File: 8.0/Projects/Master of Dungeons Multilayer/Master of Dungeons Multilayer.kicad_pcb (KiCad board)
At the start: 4 copper layers, 100 x 100 mm, 124 parts, among them J1 AudioPlug3, Q1 IRLML6244, Q10 IRLML6244, Q11 IRLML6244, Q12 IRLML6244, Q13 IRLML6244, Q14 IRLML6244, Q15 IRLML6244, Q16 IRLML6244, Q17 IRLML6244, Q2 IRLML6244, Q3 IRLML6244, Q4 IRLML6244, Q5 IRLML6244, Q6 IRLML6244, Q7 IRLML6244, Q8 IRLML6244, Q9 IRLML6244, U1 ESP32-WROOM-32E, U2 TPS63060, U3 AP2127K-3.3, U4 TSOP45xx

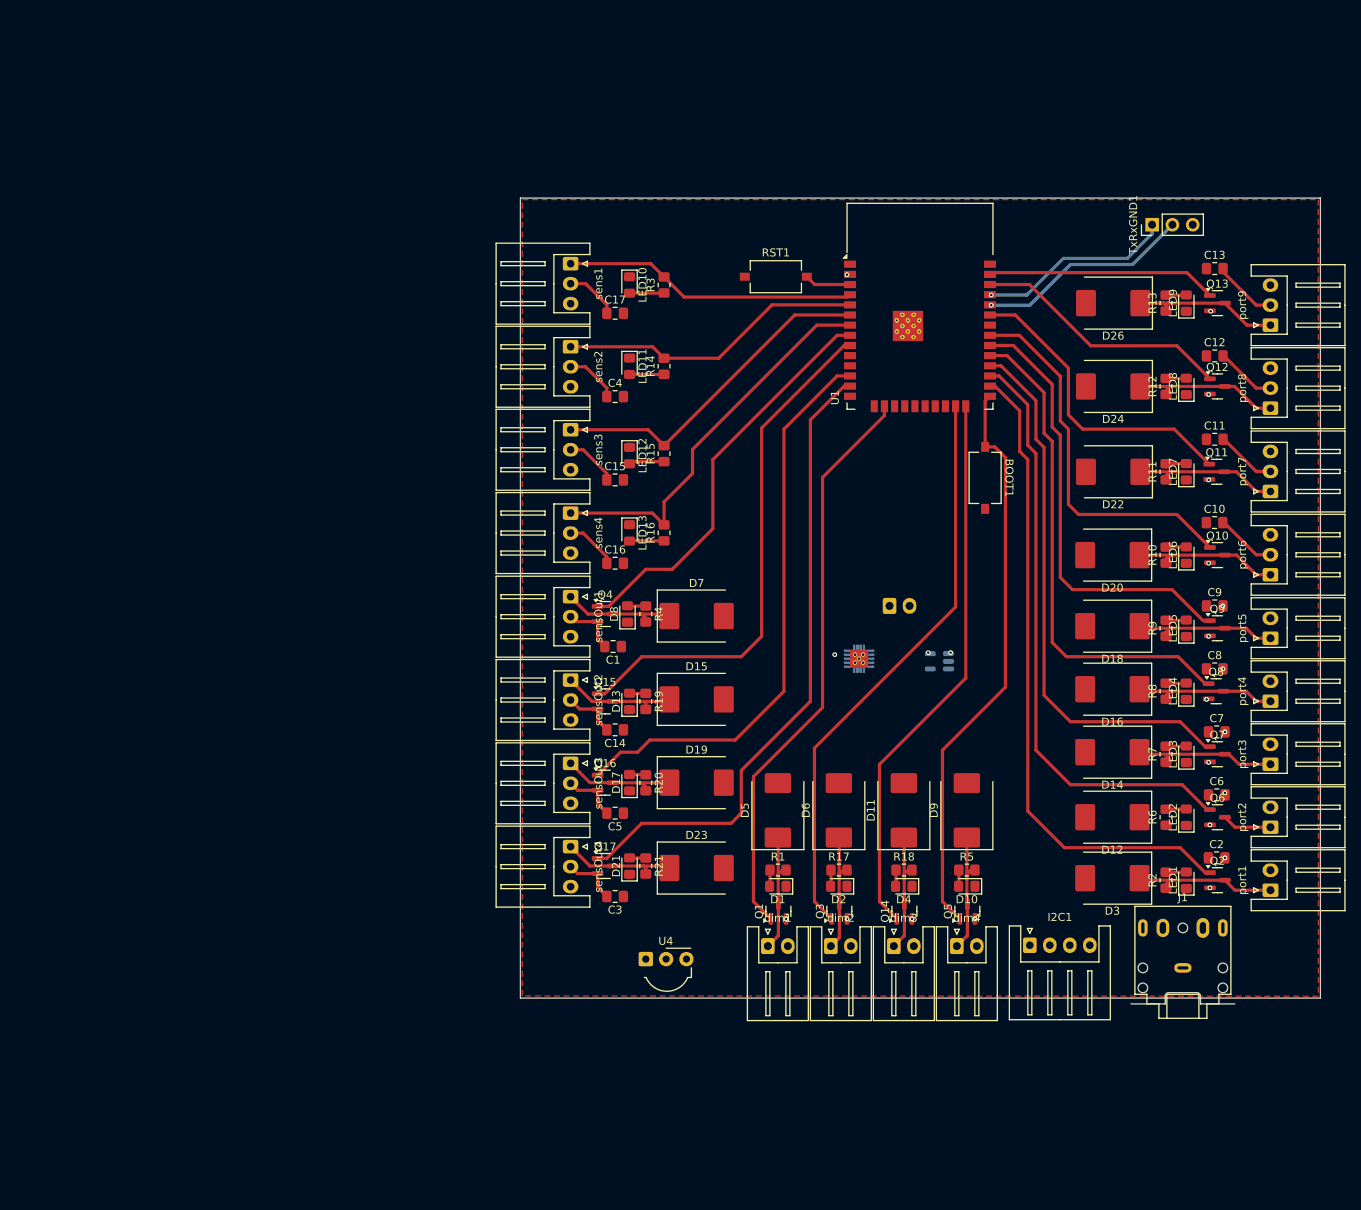
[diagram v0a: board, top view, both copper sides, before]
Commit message: update
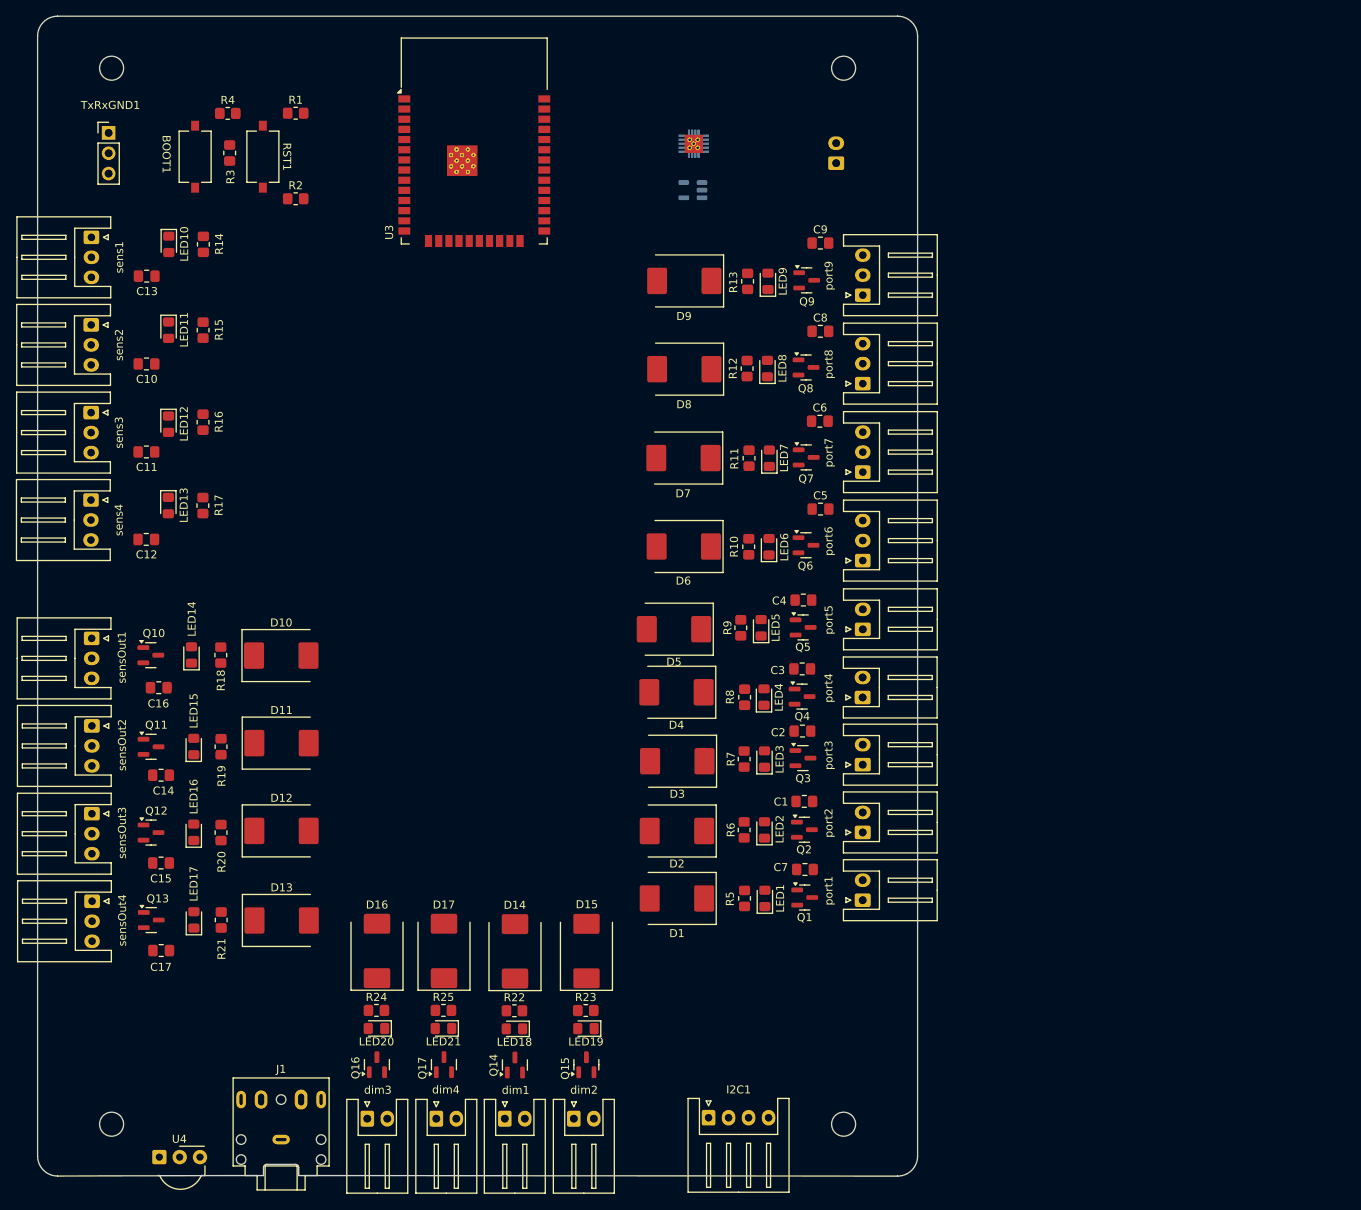
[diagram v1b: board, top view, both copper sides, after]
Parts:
- added R1: 470R, Resistor_SMD:R_0805_2012Metric_Pad1.20x1.40mm_HandSolder, F.Cu at (72.1, 39.5)
- added R2: 12K, Resistor_SMD:R_0805_2012Metric_Pad1.20x1.40mm_HandSolder, F.Cu at (72.1, 50.2)
- added R3: 12K, Resistor_SMD:R_0805_2012Metric_Pad1.20x1.40mm_HandSolder, F.Cu at (63.8, 44.5)
- added R4: 470R, Resistor_SMD:R_0805_2012Metric_Pad1.20x1.40mm_HandSolder, F.Cu at (63.6, 39.5)
- moved TxRxGND1 130.9 mm to (48.7, 42.0), turned to 0 degrees
- moved J1 114.7 mm to (70.2, 167.8)
- moved BOOT1 106.6 mm to (59.5, 44.9)
- moved U1 67.6 mm to (121.8, 43.3)
- moved U2 66.5 mm to (121.7, 49.1)
- moved RST1 65.9 mm to (68.0, 44.9), turned to -90 degrees
- moved U4 65.6 mm to (55.0, 170.0)
- moved sensOut4 60.2 mm to (46.6, 138.0)
- moved sensOut3 60.2 mm to (46.6, 127.1)
- moved sensOut2 60.1 mm to (46.6, 116.1)
- moved sensOut1 60.1 mm to (46.6, 105.2)
- moved sens2 60.0 mm to (46.5, 66.0)
- moved sens1 60.0 mm to (46.5, 55.0)
- moved sens4 60.0 mm to (46.5, 87.9)
- moved sens3 60.0 mm to (46.5, 76.9)
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- renumbered C6 to C1, C4 to C10, C15 to C11, C16 to C12, C17 to C13, C5 to C15, C1 to C16, C3 to C17, C7 to C2, C8 to C3, C9 to C4, C10 to C5, C11 to C6, C2 to C7, C12 to C8, C13 to C9, D3 to D1, D7 to D10, D15 to D11, D19 to D12, D23 to D13, D11 to D14, D9 to D15, D5 to D16, D6 to D17, D12 to D2, D14 to D3, D16 to D4, D18 to D5, D20 to D6, D22 to D7, D24 to D8, D26 to D9, D8 to LED14, D13 to LED15, D17 to LED16, D21 to LED17, D4 to LED18, D10 to LED19, D1 to LED20, D2 to LED21, Q2 to Q1, Q4 to Q10, Q15 to Q11, Q16 to Q12, Q17 to Q13, Q5 to Q15, Q1 to Q16, Q3 to Q17, Q6 to Q2, Q7 to Q3, Q8 to Q4, Q9 to Q5, Q10 to Q6, Q11 to Q7, Q12 to Q8, Q13 to Q9, R3 to R14, R14 to R15, R15 to R16, R16 to R17, R4 to R18, R18 to R22, R5 to R23, R1 to R24, R17 to R25, R2 to R5, U2 to U1, U3 to U2, U1 to U3, dim3 to dim1, dim4 to dim2, dim1 to dim3, dim2 to dim4
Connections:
- I2C1 pad 1: +5V -> GND
- I2C1 pad 2: GND -> +5V
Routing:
- net +5V: track 85.6 -> 0.00 mm, vias 19 -> 0
- net port1: track 81.4 -> 0.00 mm
- net sensOut4: track 79.7 -> 0.00 mm
- net port2: track 74.6 -> 0.00 mm
- net dim2: track 72.3 -> 0.00 mm
- net dim1: track 71.7 -> 0.00 mm
- net dim4: track 71.5 -> 0.00 mm
- net sensOut3: track 71.4 -> 0.00 mm
- net dim3: track 69.4 -> 0.00 mm
- net port3: track 68.2 -> 0.00 mm
- net sensOut2: track 64.8 -> 0.00 mm
- net port4: track 62.0 -> 0.00 mm
- net port5: track 55.3 -> 0.00 mm
- net sensOut1: track 50.6 -> 0.00 mm
- net sens4: track 49.3 -> 0.00 mm
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- removed copper zone on In2.Cu, net +3.3V
- removed copper zone on In1.Cu, net +5V
- removed copper zone on F.Cu, net GND
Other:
- board size 100 x 100 mm -> 110 x 145 mm
